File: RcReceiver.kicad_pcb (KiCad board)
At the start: 4 copper layers, 50 x 29.5 mm, 73 parts, among them J1 VBAT, J10 Servo3, J11 Servo4, J12 Servo5, J13 CAN, J14 Servo6, J15 Servo7, J16 Servo8, J17 GND for the Servo connectors, J2 SWD, J3 I2C, J4 USART1, J5 Analog input, J6 GPS, J7 SPI3, J8 Servo1, J9 Servo2, U1 LP38693-3.3, U2 STM32L476VGT6, U3 LP38693-5.0, U4 TXB0108DQSR, U5 MCP2551, U6 LP38693SD-3.3, Y1 16MHz

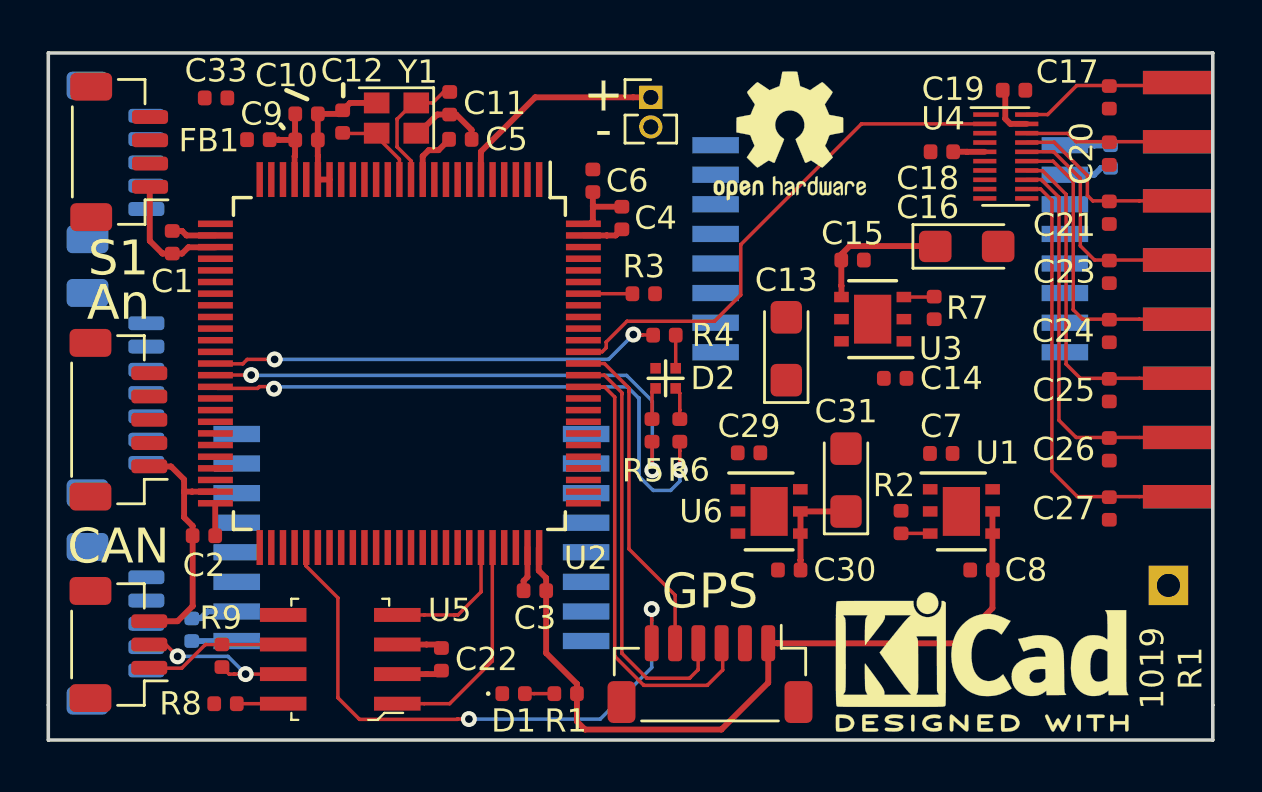
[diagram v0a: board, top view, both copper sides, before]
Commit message: More routing
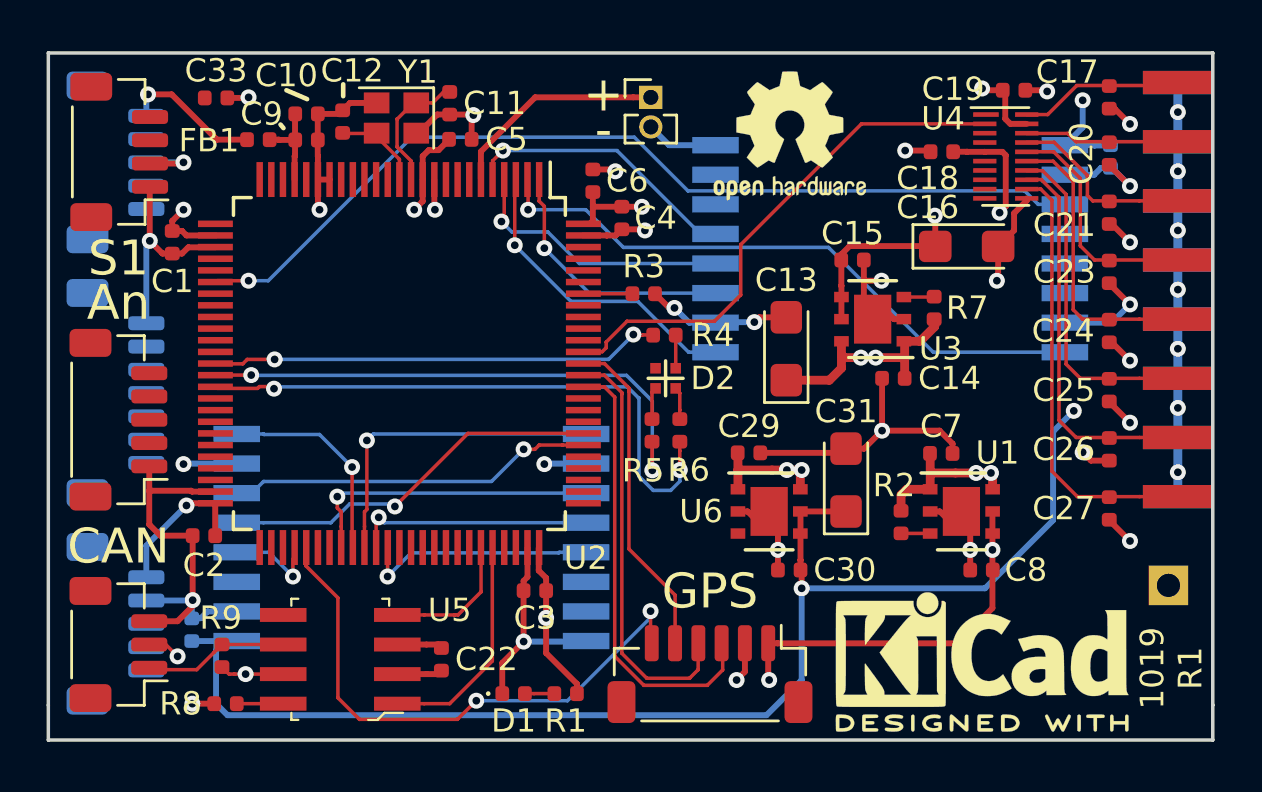
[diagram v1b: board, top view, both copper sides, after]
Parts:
- moved C14 0.08 mm to (172.3, 60.0)
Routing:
- net GND: track 31.9 -> 280.4 mm, vias 0 -> 31
- net /VCCCPU: track 47.0 -> 165.7 mm, vias 0 -> 9
- net IN: track 0.00 -> 76.4 mm, vias 0 -> 13
- net /RF modules/VCCRF: track 8.42 -> 75.3 mm, vias 0 -> 3
- net /RF1MISO: track 0.00 -> 40.2 mm, vias 0 -> 1
- net /RF1RXEN: track 0.00 -> 26.9 mm, vias 0 -> 1
- net /RF2CLK: track 0.00 -> 16.6 mm, vias 0 -> 1
- net /RF2NSS: track 0.00 -> 15.7 mm, vias 0 -> 1
- net /RF2TXEN: track 0.00 -> 14.2 mm, vias 0 -> 1
- net /RF1TXEN: track 0.00 -> 13.4 mm, vias 0 -> 1
- net /RF2NRESET: track 0.00 -> 13.0 mm, vias 0 -> 1
- net /RF1IRQ: track 0.00 -> 12.0 mm, vias 0 -> 1
- net /RF1BUSY: track 0.00 -> 11.9 mm, vias 0 -> 1
- net /RF1NRESET: track 0.00 -> 11.2 mm, vias 0 -> 1
- net /RF2BUSY: track 0.00 -> 10.3 mm, vias 0 -> 1
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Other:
- net class IN: via_dia 1.016 -> 0.6858; via_drill 0.6 -> 0.3302
- net class VCC: via_dia 1.016 -> 0.6858; via_drill 0.6 -> 0.3302
